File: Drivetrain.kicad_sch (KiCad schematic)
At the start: 91 parts, among them J501 Conn_01x03, J502 SWD, J503 Conn_01x13, J504 Conn_01x06, J505 Conn_01x06, J506 CAN_A_PROBE, J507 CAN_B_PROBE, SW501 SW_Push, SW502 219-2MSTR, SW503 219-2MSTR, SW504 CVS-01TB, SW505 CVS-01TB, U501 STM32F401RETx, U502 L298P, U503 ACS712xLCTR-05B, U504 MCP2515T-I/ST, U505 MCP2515T-I/ST, U506 ACS712xLCTR-05B, U507 SN65HVD230DR, U508 SN65HVD230DR, Y501 16 MHz, Y502 16 MHz

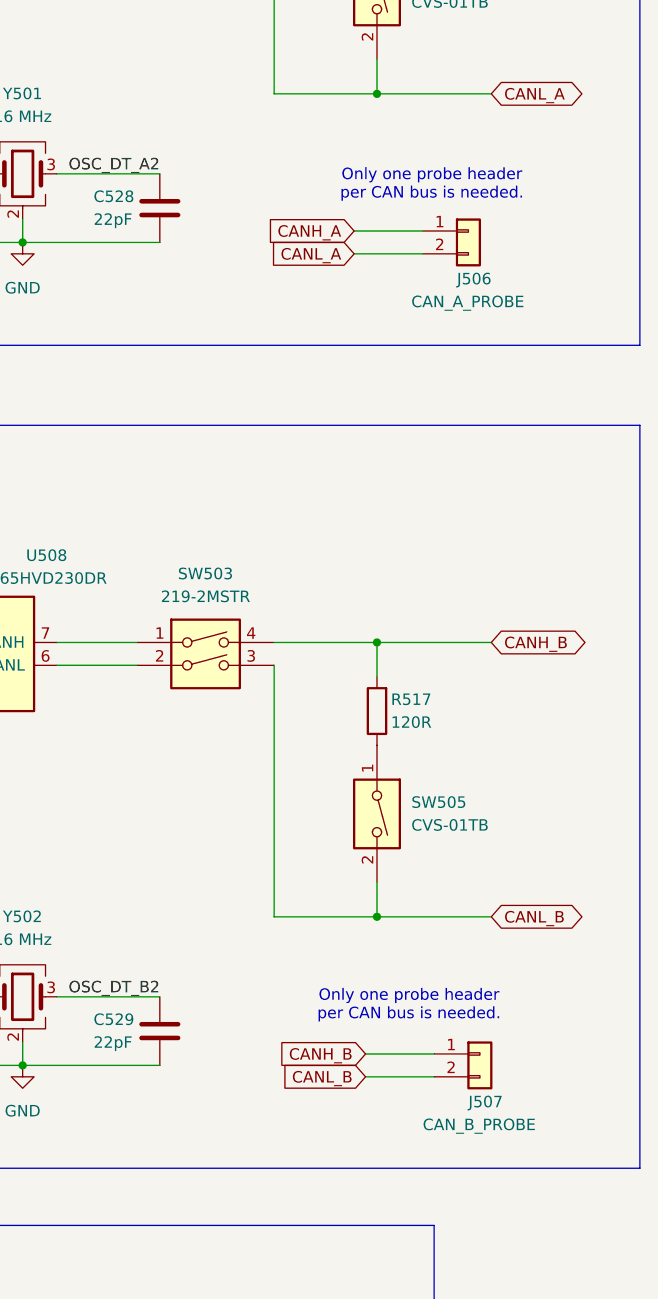
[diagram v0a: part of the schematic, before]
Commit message: started layout
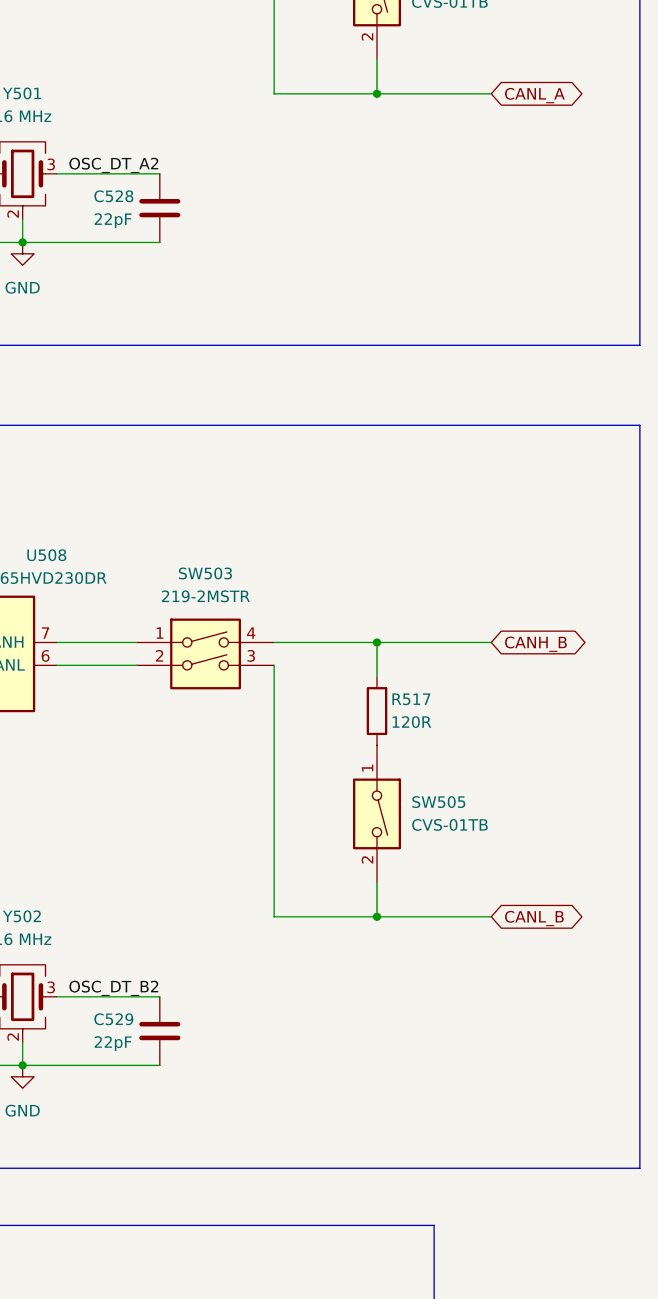
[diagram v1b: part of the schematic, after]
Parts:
- removed J506: CAN_A_PROBE, Connector_PinHeader_2.54mm:PinHeader_1x02_P2.54mm_Vertical, symbol Connector_Generic:Conn_01x02
- removed J507: CAN_B_PROBE, Connector_PinHeader_2.54mm:PinHeader_1x02_P2.54mm_Vertical, symbol Connector_Generic:Conn_01x02
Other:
- note removed: "Only one probe header per CAN bus is needed."

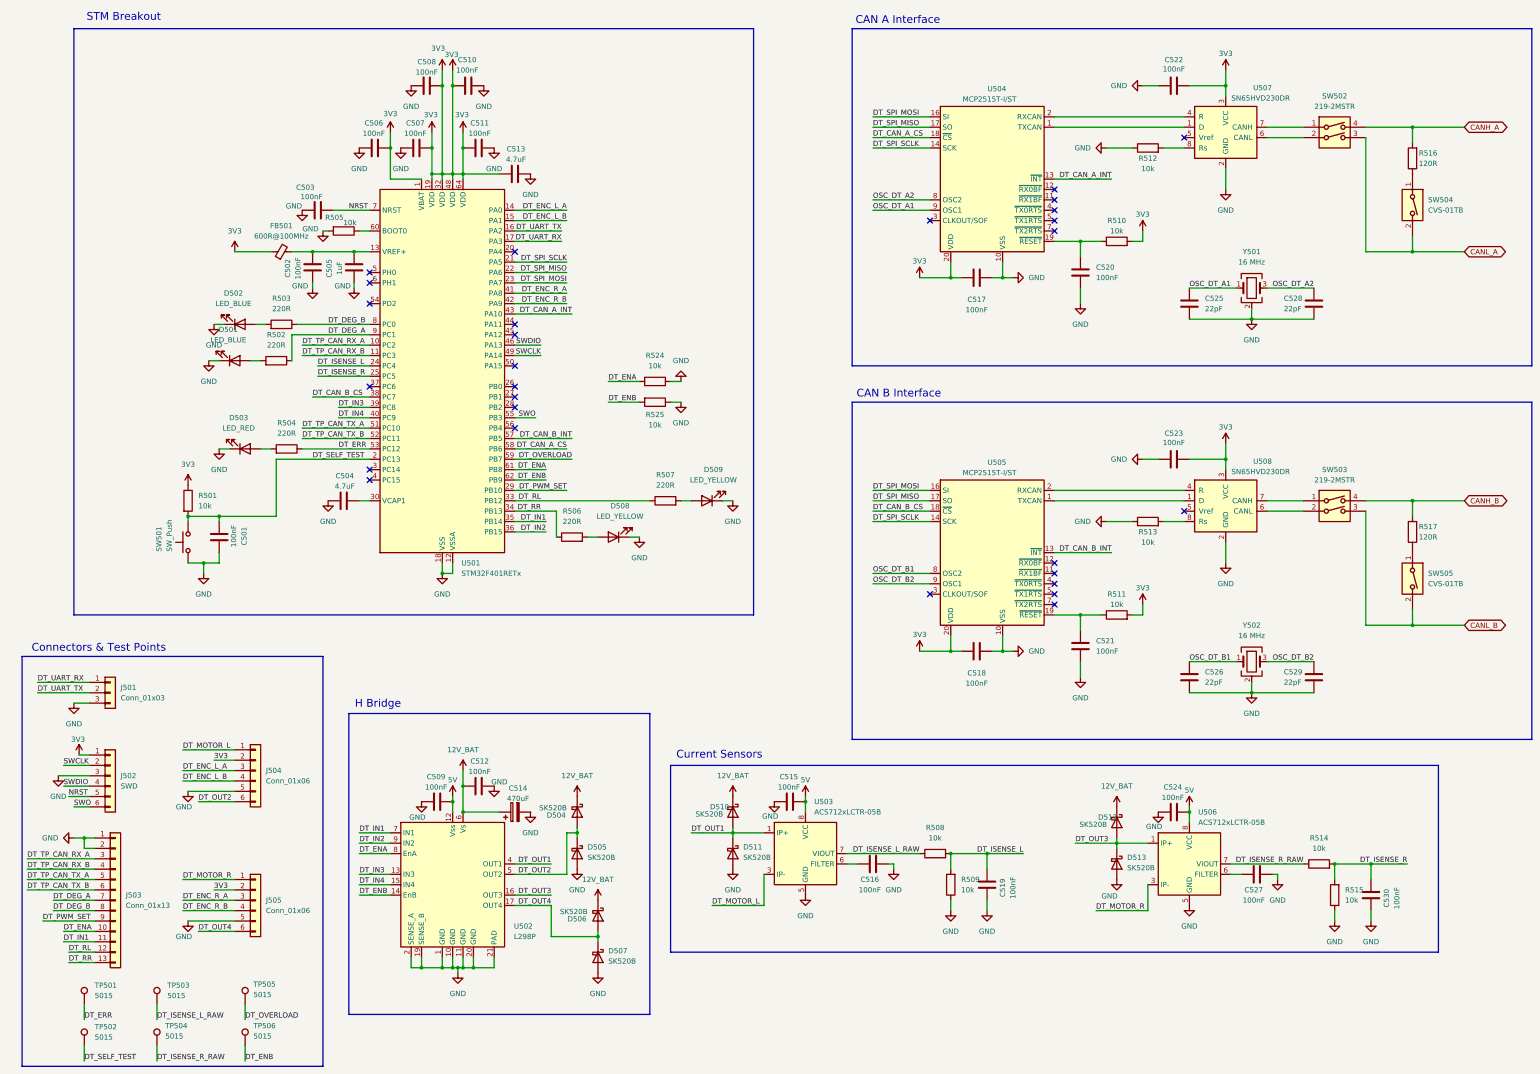
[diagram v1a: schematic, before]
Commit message: DT layout done
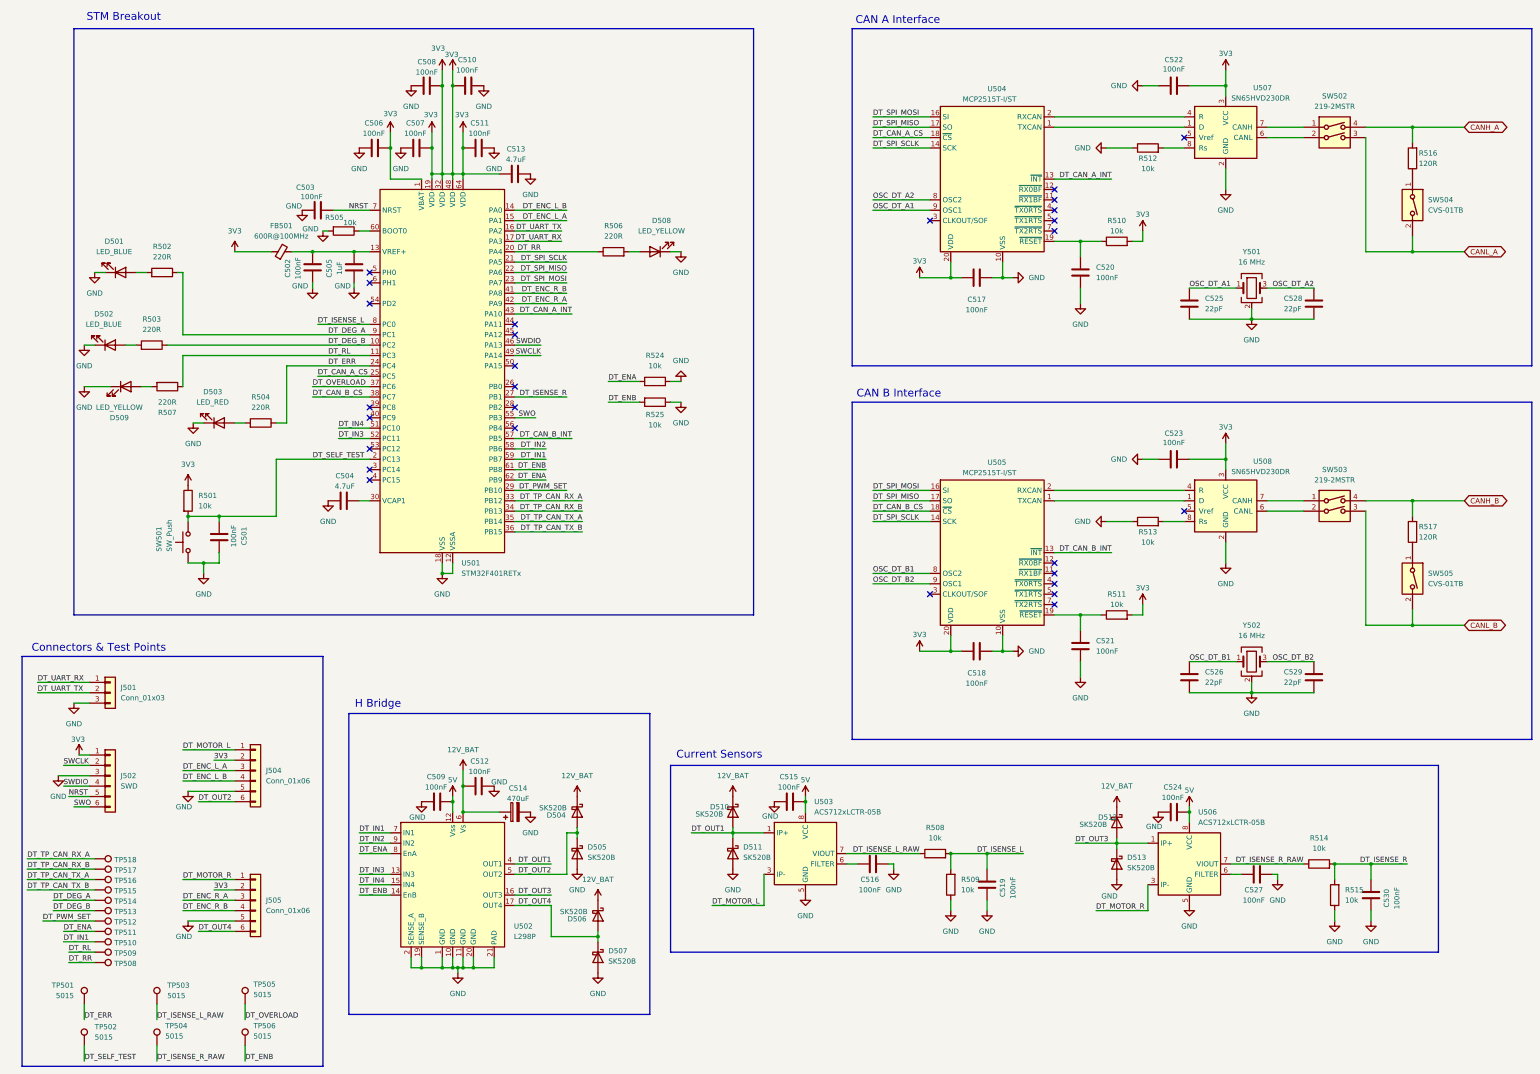
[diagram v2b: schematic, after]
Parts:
- removed J503: Conn_01x13, Connector_PinHeader_2.54mm:PinHeader_1x13_P2.54mm_Vertical, symbol Connector_Generic:Conn_01x13
- added TP508, TP509, TP510, TP511, TP512, TP513, TP514, TP515, TP516, TP517, TP518: 5015, TestPoint:TestPoint_Keystone_5015_Micro_Mini, symbol Connector:TestPoint
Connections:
- net DT_CAN_A_CS: now also U501.25 (PC5); no longer U501.58 (PB6)
- net DT_DEG_A: now also TP514.1
- net DT_DEG_B: now also U501.10 (PC2), TP513.1; no longer U501.8 (PC0)
- net DT_ENA: now also U501.62 (PB9), TP511.1; no longer U501.61 (PB8)
- net DT_ENB: now also U501.61 (PB8); no longer U501.62 (PB9)
- net DT_ENC_L_A: now also U501.15 (PA1); no longer U501.14 (PA0)
- net DT_ENC_L_B: now also U501.14 (PA0); no longer U501.15 (PA1)
- net DT_ENC_R_A: now also U501.42 (PA9); no longer U501.41 (PA8)
- net DT_ENC_R_B: now also U501.41 (PA8); no longer U501.42 (PA9)
- net DT_ERR: now also U501.24 (PC4); no longer U501.53 (PC12)
- net DT_IN1: now also U501.59 (PB7), TP510.1; no longer U501.35 (PB14)
- net DT_IN2: now also U501.58 (PB6); no longer U501.36 (PB15)
- net DT_IN3: now also U501.52 (PC11); no longer U501.39 (PC8)
- net DT_IN4: now also U501.51 (PC10); no longer U501.40 (PC9)
- net DT_ISENSE_L: now also U501.8 (PC0); no longer U501.24 (PC4)
- net DT_ISENSE_R: now also U501.27 (PB1); no longer U501.25 (PC5)
- net DT_OVERLOAD: now also U501.37 (PC6); no longer U501.59 (PB7)
- net DT_PWM_SET: now also TP512.1
- net DT_RL: now also U501.11 (PC3), TP509.1; no longer U501.33 (PB12)
- net DT_RR: now also U501.20 (PA4), TP508.1; no longer U501.34 (PB13)
- net DT_TP_CAN_RX_A: now also U501.33 (PB12), TP518.1; no longer U501.10 (PC2)
- net DT_TP_CAN_RX_B: now also U501.34 (PB13), TP517.1; no longer U501.11 (PC3)
- net DT_TP_CAN_TX_A: now also U501.35 (PB14), TP516.1; no longer U501.51 (PC10)
- net DT_TP_CAN_TX_B: now also U501.36 (PB15), TP515.1; no longer U501.52 (PC11)
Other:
- moved on the sheet: D501, R502
